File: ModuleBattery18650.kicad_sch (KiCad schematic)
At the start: 25 parts, among them J1 Connector_6p, T1 SISH615ADN, T2 SISH615ADN, T3 FDN337N, T4 SISH615ADN, T5 SISH615ADN, U1 MCP121T-315E

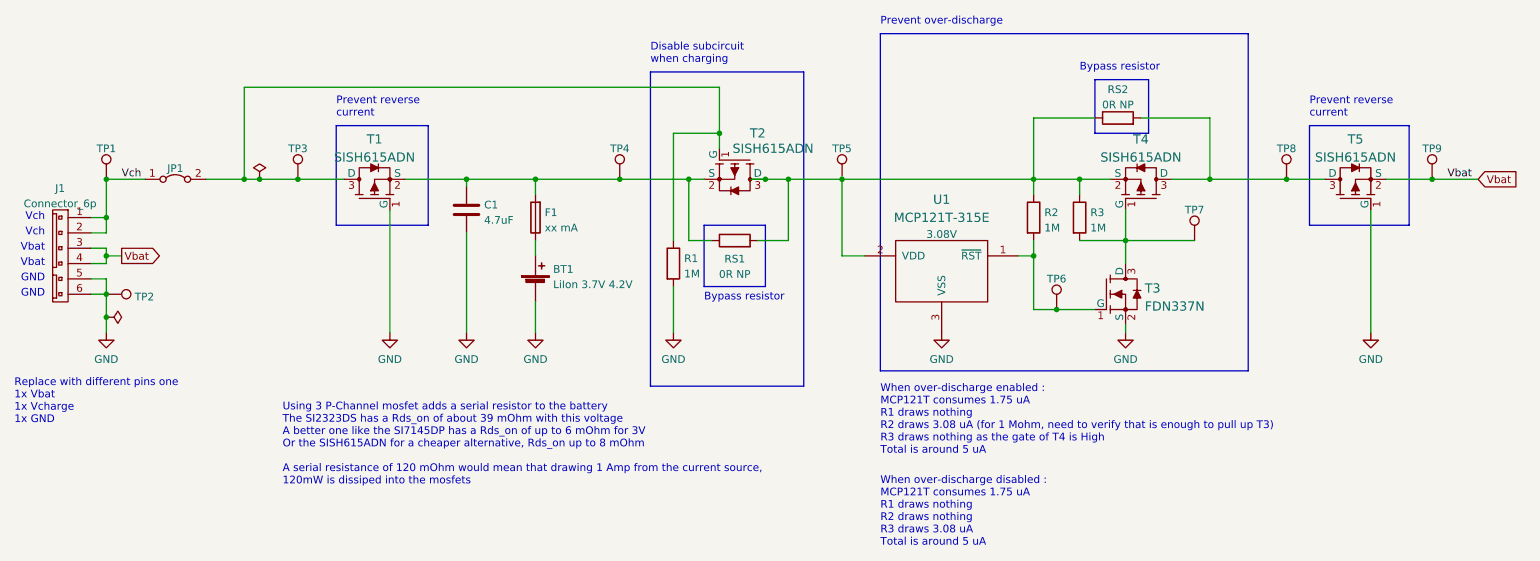
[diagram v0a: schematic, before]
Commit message: adapted footprints
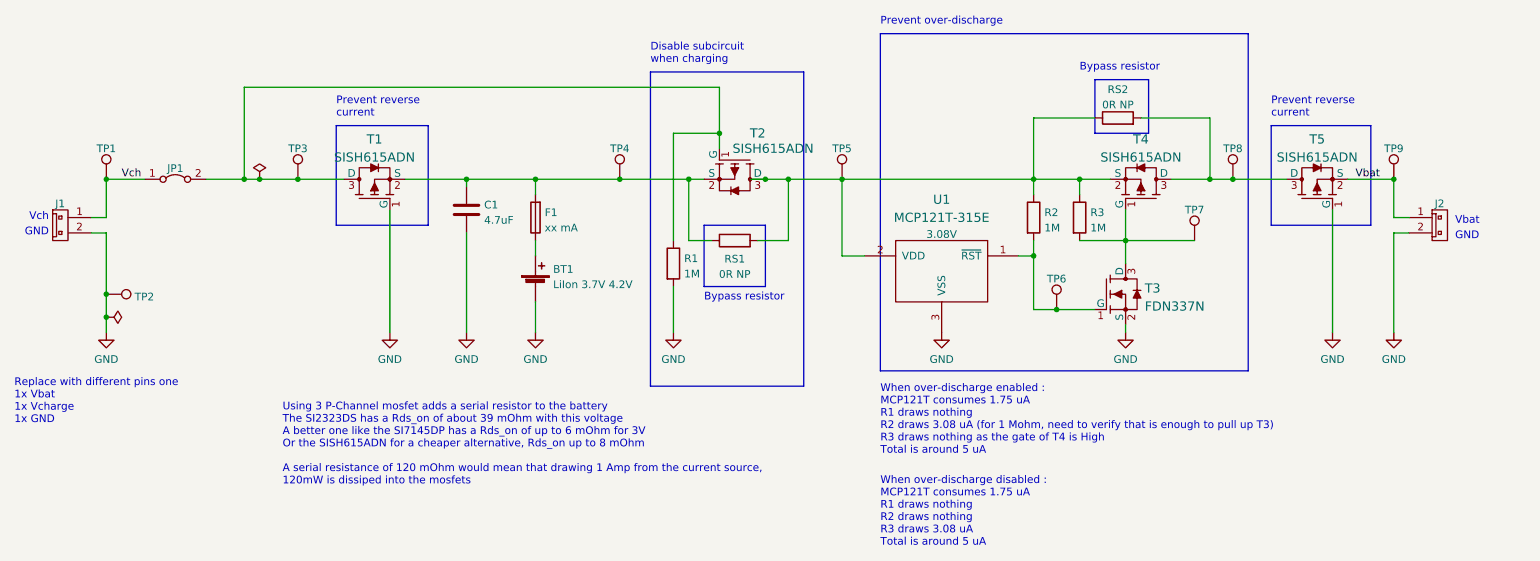
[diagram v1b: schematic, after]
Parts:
- removed J1: Connector_6p, 0ESN_Lib:Connector_6p_m, symbol 0ESN_Lib:Connector_6p
- added J1: Connector_2p, 0ESN_Lib:Connector_2p_m, symbol 0ESN_Lib:Connector_2p
- added J2: Connector_2p_r, 0ESN_Lib:Connector_2p_m, symbol 0ESN_Lib:Connector_2p_r
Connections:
- net GND: now also J1.2 (P2), J2.2 (P2)
- net Vbat: now also J2.1 (P1)
- net Vch: now also J1.1 (P1)
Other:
- moved on the sheet: T5, TP8, TP9
